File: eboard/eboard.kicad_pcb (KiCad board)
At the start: 4 copper layers, 90.3 x 95.8 mm, 132 parts, among them J1 Conn_01x02_Male, J10 Conn_01x06_Male, J11 Conn_01x02_Male, J12 Conn_01x02_Male, J13 Conn_01x02_Male, J14 Conn_01x02_Male, J15 Conn_01x02_Male, J16 Conn_01x03_Male, J17 Conn_01x03_Male, J18 Conn_01x03_Male, J19 Conn_01x03_Male, J2 USB_B_Micro, J20 Conn_01x02_Male, J21 Conn_01x03_Male, J3 Conn_01x03_Male, J4 jst_battery, J5 Conn_01x02_Male, J6 Conn_01x03_Male, J7 Conn_01x04_Male, J8 Conn_01x04_Male, J9 Conn_01x06_Male, Q1 AO4407A_new, Q10 BSS138K, Q11 AO4407A_new, Q12 BSS138K, Q13 BSS138K, Q14 BSS138K, Q15 BSS138K, Q16 BSS138K, Q17 BSS138K, Q18 AO4407A_new, Q19 AO4407A_new, Q2 S8050, Q20 AO4407A_new, Q3 S8050, Q4 BSS138K, Q5 BSS138K, Q6 AO4407A_new, Q7 BSS138K, Q8 BSS138K, Q9 BSS138K, SW1 pushbutton_switch, SW2 pushbutton_switch, U1 ESP32-PICO-D4, U2 TPS63000, U3 TP4056, U4 SRV05-4, U5 CP2102, U6 TPS63000, U7 SRV05-4, U8 SRV05-4, U9 SRV05-4

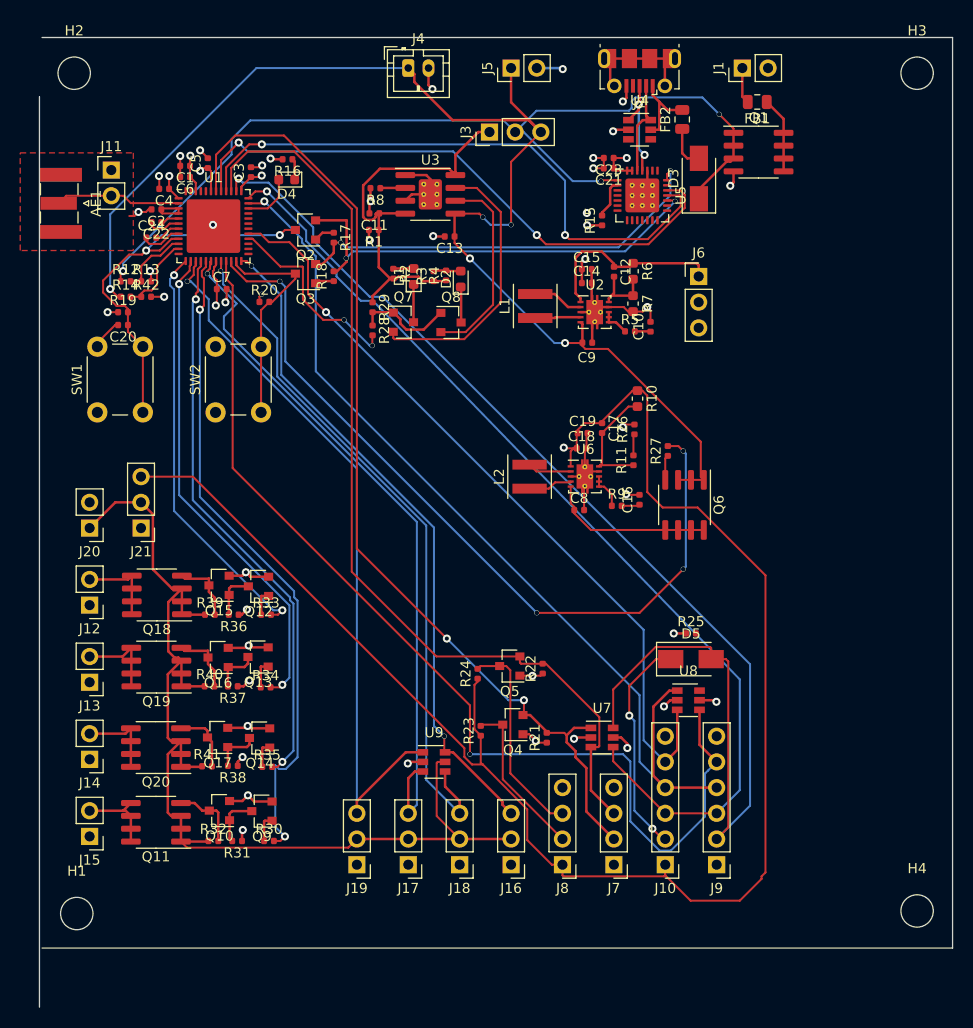
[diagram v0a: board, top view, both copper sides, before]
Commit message: routed
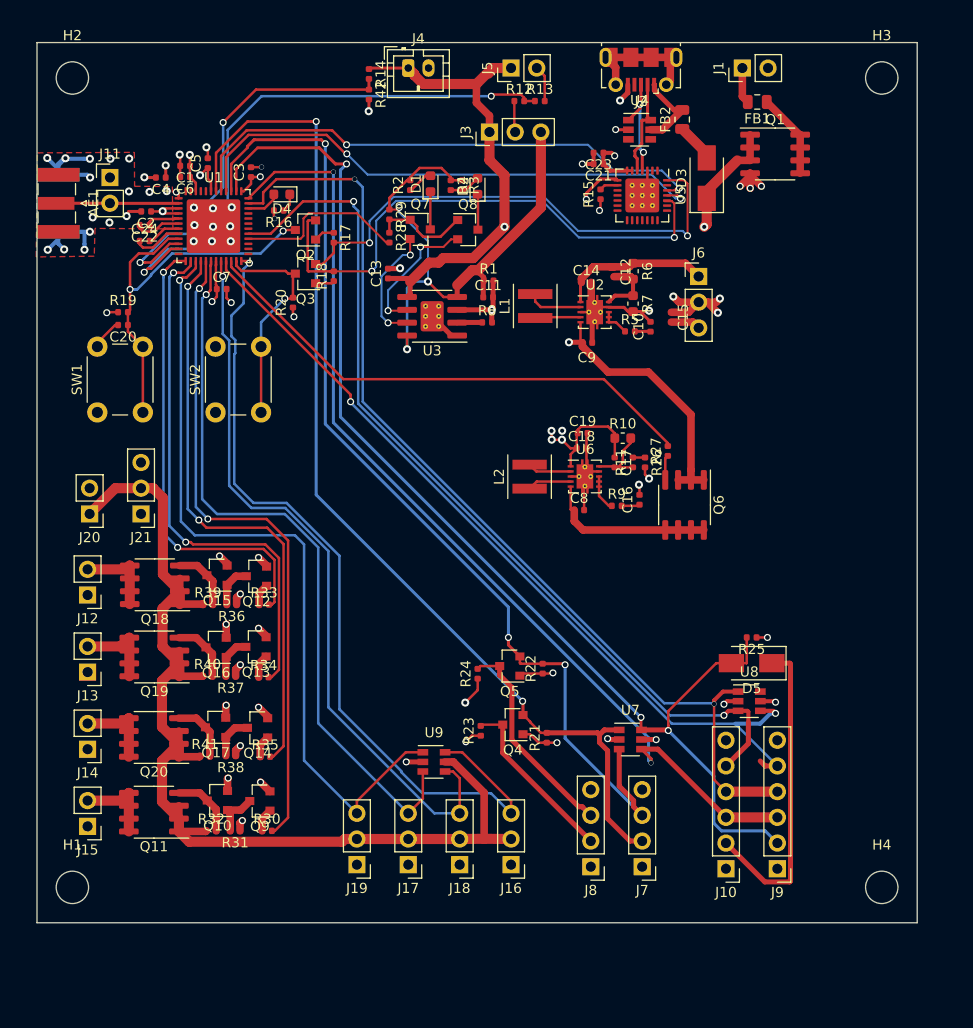
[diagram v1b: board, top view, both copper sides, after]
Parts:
- moved R12 42.8 mm to (87.2, 36.3)
- moved R13 42.8 mm to (89.2, 36.3)
- moved R14 32.6 mm to (72.3, 33.6), turned to 270 degrees
- moved R42 29.7 mm to (72.3, 35.6), turned to 270 degrees
- moved R8 17.3 mm to (84.0, 58.2), turned to 0 degrees
- moved C11 14.0 mm to (84.1, 55.7), turned to 0 degrees
- moved R1 12.4 mm to (84.1, 54.0), turned to 0 degrees
- moved U3 12.1 mm to (78.6, 57.6), turned to 180 degrees
- moved C15 9.61 mm to (102.2, 57.6), turned to 270 degrees
- moved R3 9.42 mm to (81.5, 44.6), turned to 270 degrees
- moved Q7 9.32 mm to (77.4, 49.0)
- moved R28 9.32 mm to (74.3, 49.8)
- moved R29 9.32 mm to (74.3, 47.5)
- moved Q8 9.32 mm to (82.1, 49.0)
- moved D1 9.32 mm to (78.4, 44.4)
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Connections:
- C14 pad 1: +3V3 -> Net-(C12-Pad1)
- J3 pad 1: Vcharge -> Vraw
- J3 pad 3: Vraw -> Vcharge
- U1 pad 10: ADC0 -> ADC1
- U1 pad 11: ADC1 -> ADC0
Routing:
- net ADC0: track 7.18 -> 56.9 mm, vias 0 -> 2
- net Vin: track 93.3 -> 43.8 mm, vias 3 -> 2
- net Vraw: track 128.4 -> 89.1 mm, vias 5 -> 2
- net ADC1: track 7.99 -> 40.3 mm, vias 0 -> 2
- net +5V: track 161.6 -> 130.2 mm, vias 1 -> 6
- net DISABLE_5v: track 79.1 -> 51.2 mm, vias 4 -> 0
- net SPI_CS0: track 102.5 -> 83.8 mm, vias 1 -> 2
- net GND: track 96.0 -> 113.3 mm, vias 31 -> 54
- net IO0: track 66.4 -> 83.1 mm, vias 2 -> 1
- net Vcharge: track 40.0 -> 56.2 mm, vias 0 -> 3
- net nCHRG: track 27.2 -> 12.1 mm, vias 0 -> 2
- net SPI_CS1: track 76.8 -> 89.9 mm, vias 1 -> 2
- net MISO_5v: track 21.9 -> 31.3 mm, vias 2 -> 0
- net MISO: track 127.3 -> 118.1 mm, vias 1 -> 3
- net +3V3: track 46.7 -> 56.0 mm, vias 19 -> 23
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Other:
- board size 90.3 x 95.8 mm -> 87 x 87 mm
